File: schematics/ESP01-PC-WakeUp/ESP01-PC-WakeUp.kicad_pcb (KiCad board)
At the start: 2 copper layers, 18 parts, among them J1 JUSB, J2 JUSB, J3 Pin selector, J4 Power, J5 Out 1, J6 Out 2, Q1 BC337, Q2 2N7000, U1 ESP-01, U2 PS2561

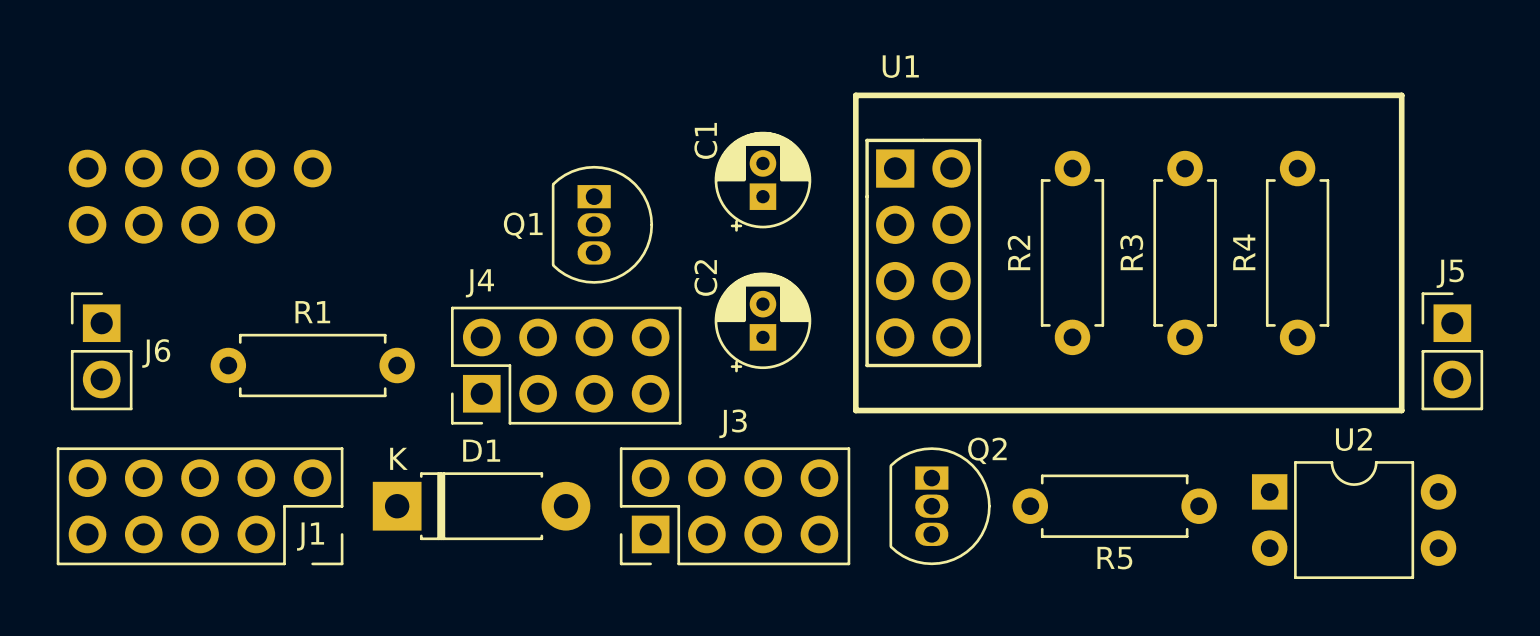
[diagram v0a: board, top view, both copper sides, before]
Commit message: feat: first PCB release.
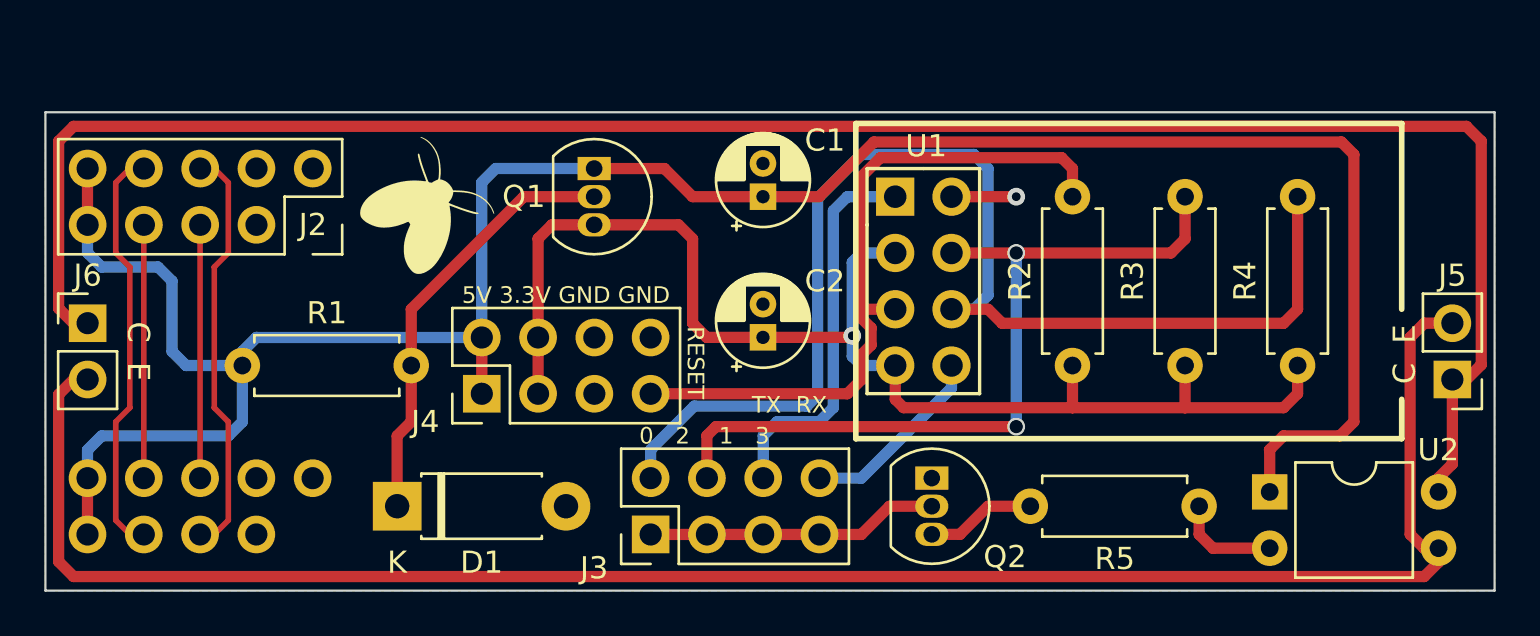
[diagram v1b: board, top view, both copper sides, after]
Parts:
- J1: moved to B.Cu
- J2: moved to F.Cu
- moved J1 5.08 mm to (182.9, 92.7), turned to 90 degrees
- moved J2 2.54 mm to (182.9, 76.2), turned to -90 degrees
- moved J5 2.54 mm to (234.3, 85.7), turned to 180 degrees
- moved R2 1.27 mm to (217.2, 85.1)
- moved R3 1.27 mm to (222.2, 85.1)
- moved R4 1.27 mm to (227.3, 85.1)
- moved Q1 1.27 mm to (195.6, 76.2)
- moved U1 1.27 mm to (209.2, 77.5)
- moved R1 0.64 mm to (179.7, 85.1)
- moved J6 0.63 mm to (172.7, 83.2)
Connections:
- J1 pad 5: D+ -> D2+
- J1 pad 6: D+ -> D1+
- J1 pad 7: D- -> D2-
- J1 pad 8: D- -> D1-
- J2 pad 5: D+ -> D1+
- J2 pad 6: D+ -> D2+
- J2 pad 7: D- -> D1-
- J2 pad 8: D- -> D2-
- J3 pad 1: 0 -> PW
- J3 pad 2: PW -> 0
- J3 pad 3: 2 -> PW
- J3 pad 4: PW -> 2
- J3 pad 5: TX -> PW
- J3 pad 6: PW -> TX
- J3 pad 7: RX -> PW
- J3 pad 8: PW -> RX
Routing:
- net +5V: track 0.00 -> 109.6 mm
- net Net-(J5-Pad1): track 0.00 -> 90.9 mm
- net Net-(J5-Pad2): track 0.00 -> 85.2 mm
- net +3V3: track 0.00 -> 59.5 mm, vias 0 -> 1
- net 0: track 0.00 -> 56.4 mm
- net 2: track 0.00 -> 36.6 mm, vias 0 -> 2
- net RST: track 0.00 -> 32.2 mm
- net Net-(D1-Pad1): track 0.00 -> 19.5 mm
- net D2+: track 0.00 -> 18.8 mm
- net D2-: track 0.00 -> 18.8 mm
- net TX: track 0.00 -> 17.6 mm
- net PW: track 0.00 -> 13.2 mm
- net D1-: track 0.00 -> 11.4 mm
- net D1+: track 0.00 -> 11.4 mm
- net RX: track 0.00 -> 8.66 mm
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- added copper zone on B.Cu, net GND
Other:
- board outline added: 65.4 x 21.6 mm
- board text added: "0 2 1 3"
- board text added: "5V 3.3V GND GND"
- board text added: "C E"
- board text added: "RESET"
- board text added: "TX RX"
